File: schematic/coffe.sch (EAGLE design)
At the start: 18 parts, among them Q1 BC546B

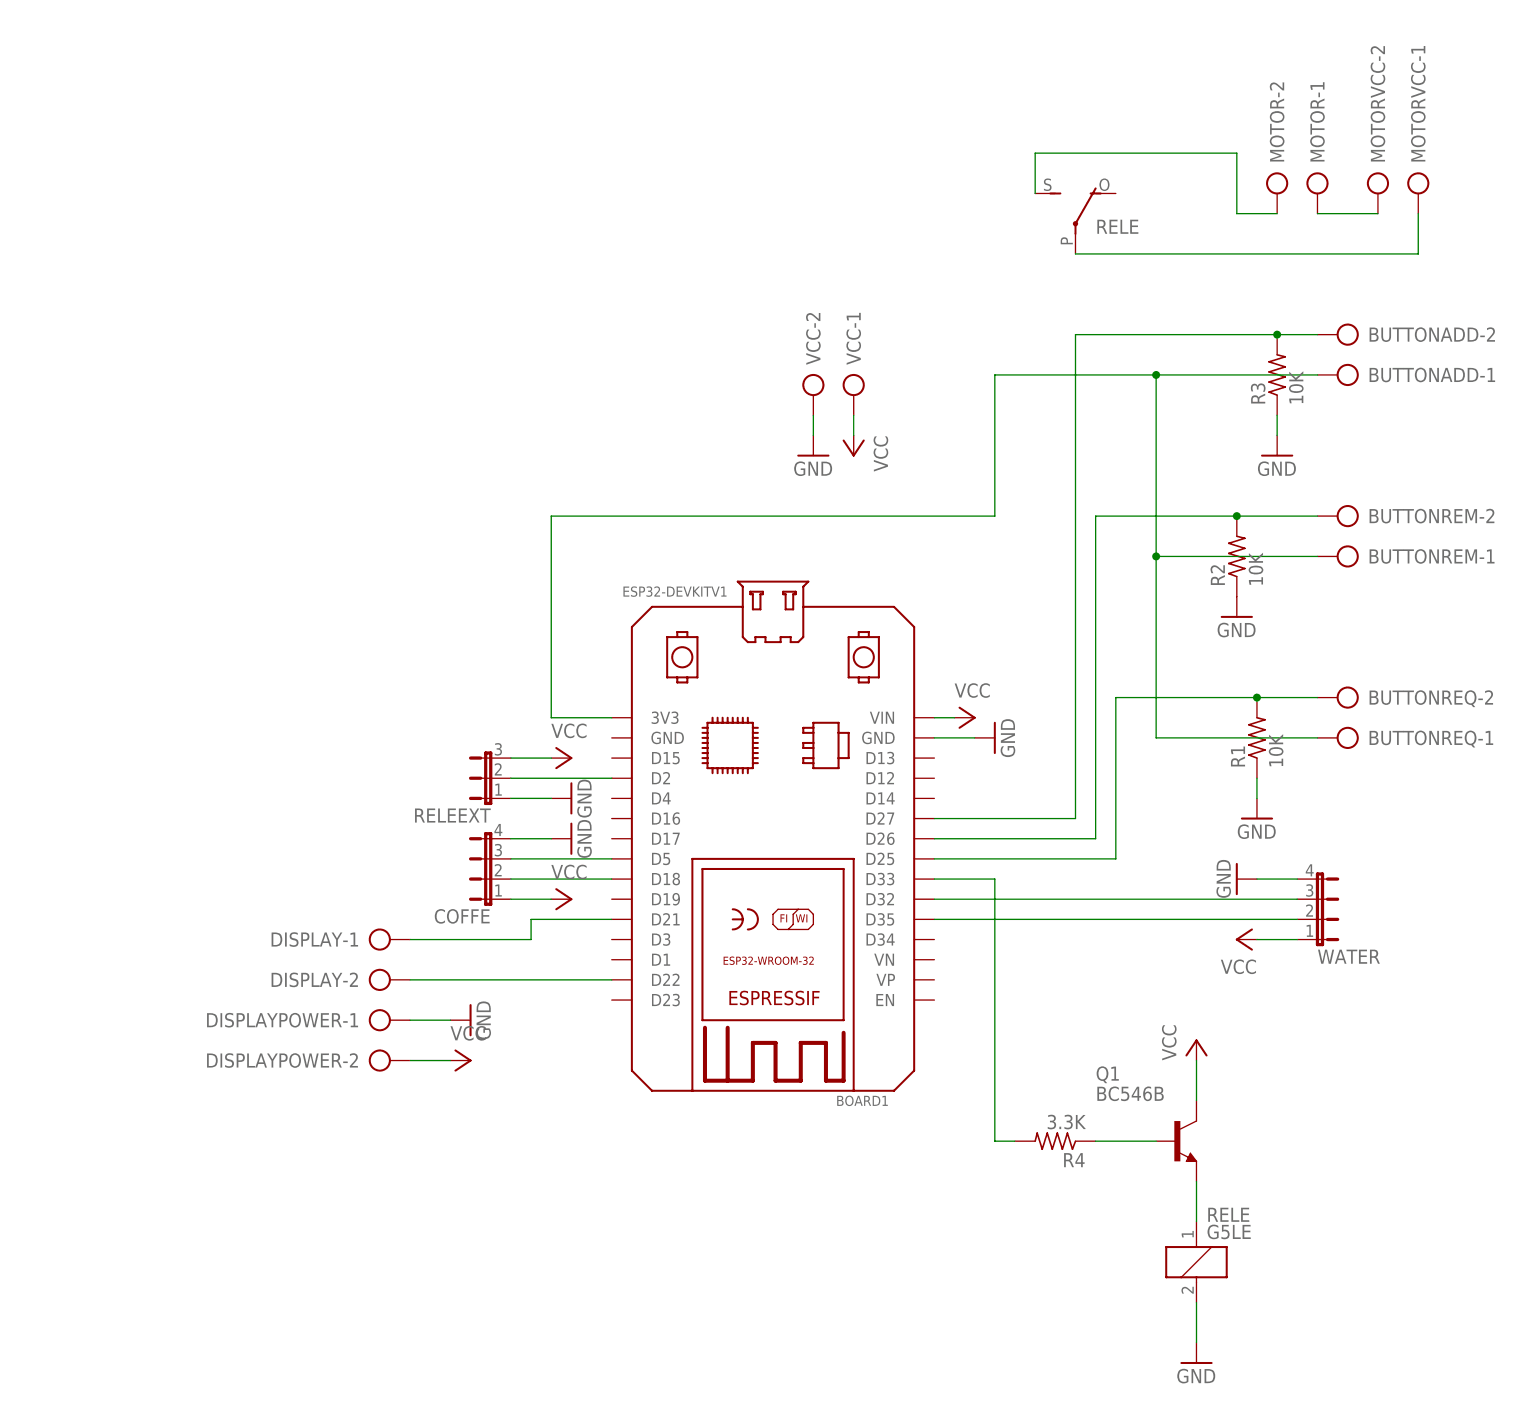
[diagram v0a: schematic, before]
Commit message: Routing complete
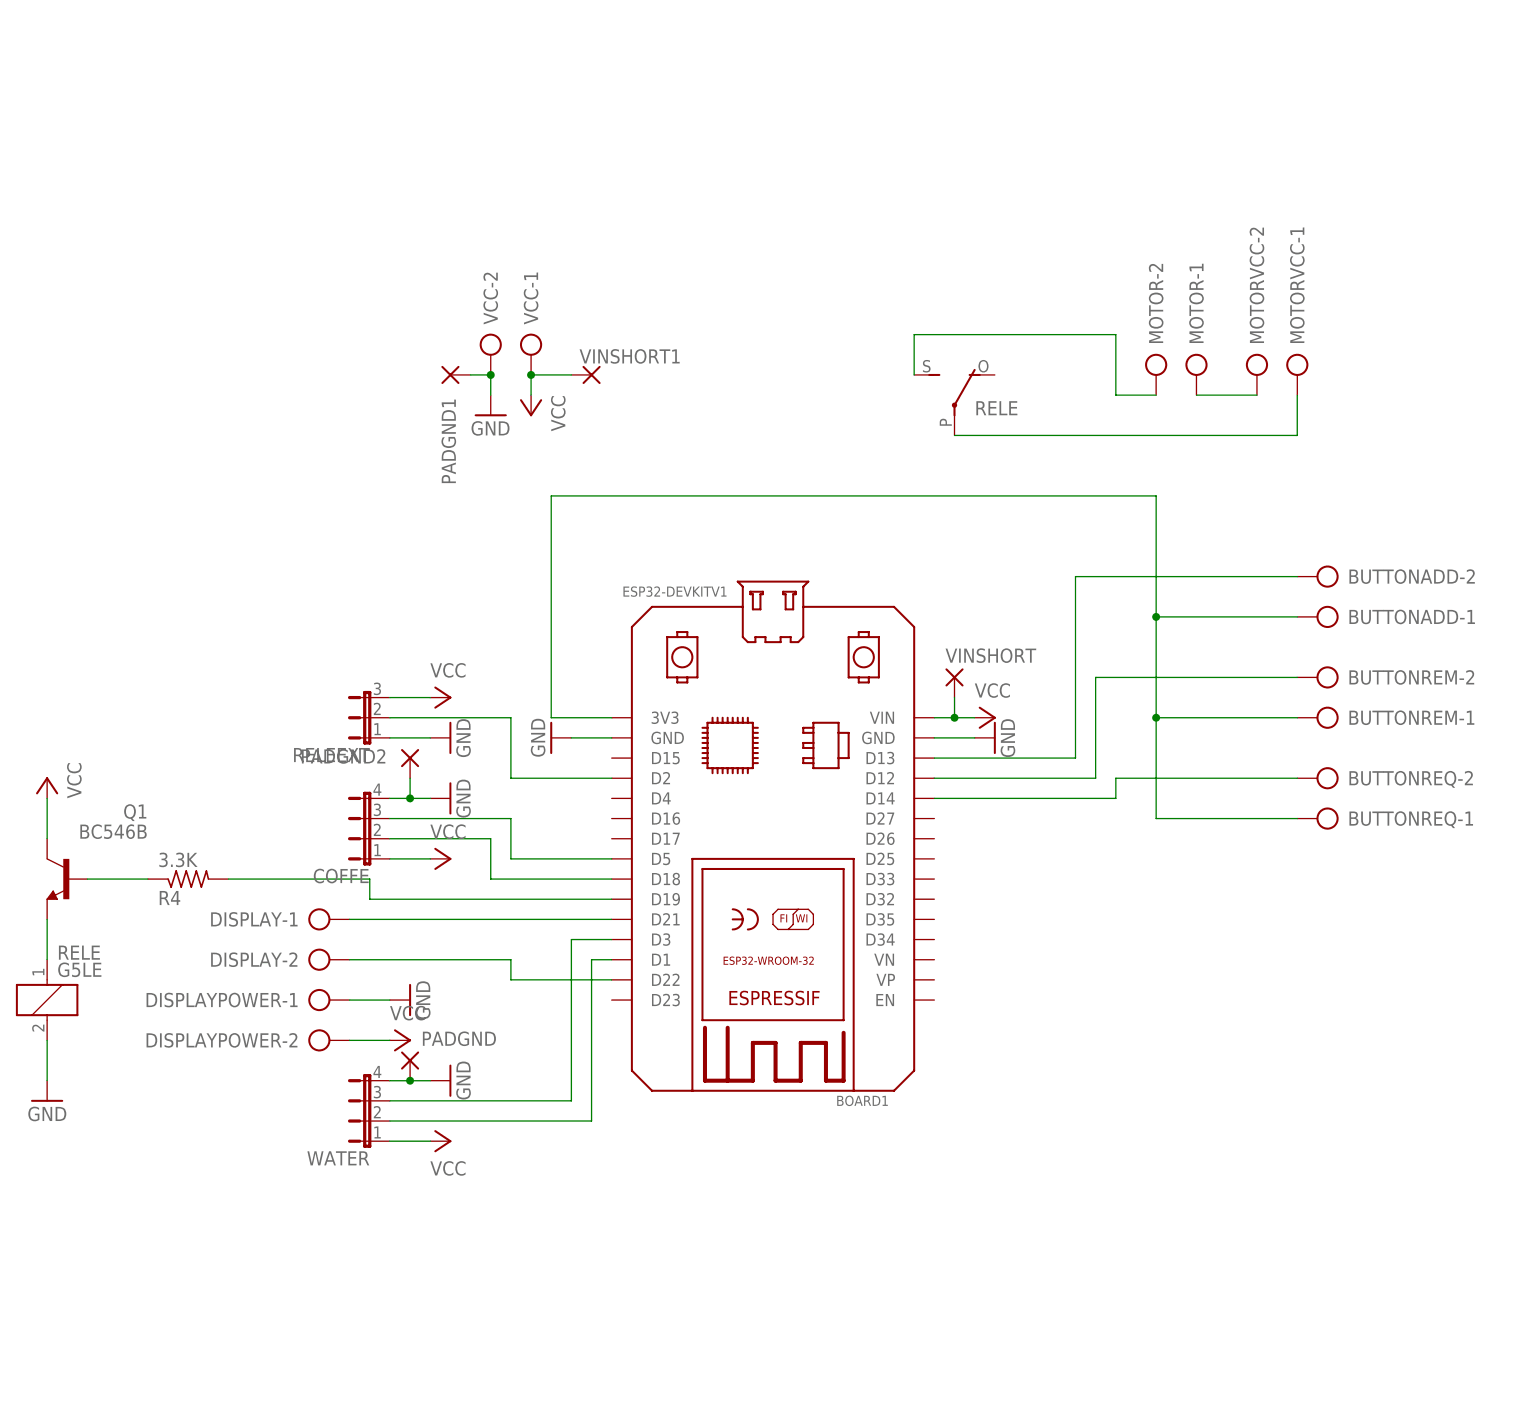
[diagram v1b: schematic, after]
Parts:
- removed R1, R2, R3: 10K, rcl:R-US_0204/7
- added PADGND, PADGND1, PADGND2, VINSHORT, VINSHORT1: (no value), wirepad:2,15/1,0
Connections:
- removed net N$7 (its old number): BOARD1.D33, R4.2
- new net N$5: BOARD1.D14, BUTTONREQ-2.KL
- net GND: now also BOARD1.GND@1, PADGND.P, PADGND1.P, PADGND2.P; no longer R1.1, R2.1, R3.1
- net N$1: now also BOARD1.D3; no longer BOARD1.D32
- net N$16: now also BOARD1.D13; no longer BOARD1.D27, R3.2
- net N$18: now also BOARD1.D12; no longer BOARD1.D26, R2.2
- net N$2: now also BOARD1.D1; no longer BOARD1.D35
- net N$6: now also BOARD1.D19, R4.2; no longer BOARD1.D25, BUTTONREQ-2.KL, R1.2
- net VCC: now also VINSHORT.P, VINSHORT1.P
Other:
- moved on the sheet: BUTTONADD-1, BUTTONADD-2, BUTTONREM-1, BUTTONREM-2, BUTTONREQ-1, BUTTONREQ-2, COFFE, DISPLAY-1, DISPLAY-2, DISPLAYPOWER-1, DISPLAYPOWER-2, MOTOR-1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
